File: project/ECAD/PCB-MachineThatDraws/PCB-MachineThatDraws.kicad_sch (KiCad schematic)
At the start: 29 parts, among them J1 SD_Card_Device, J10 Conn_02x03_Odd_Even, J11 Conn_02x03_Odd_Even, J2 SDA/SCL/VCC/GND, J3 Switch, J4 Limit_Switch_X, J5 Moteur, J6 Moteur, J7 Barrel_Jack_Switch, J8 Screw_Terminal_01x02, J9 Servo, U1 ESP32-S3-UNO, U2 R-78E5.0-1.0

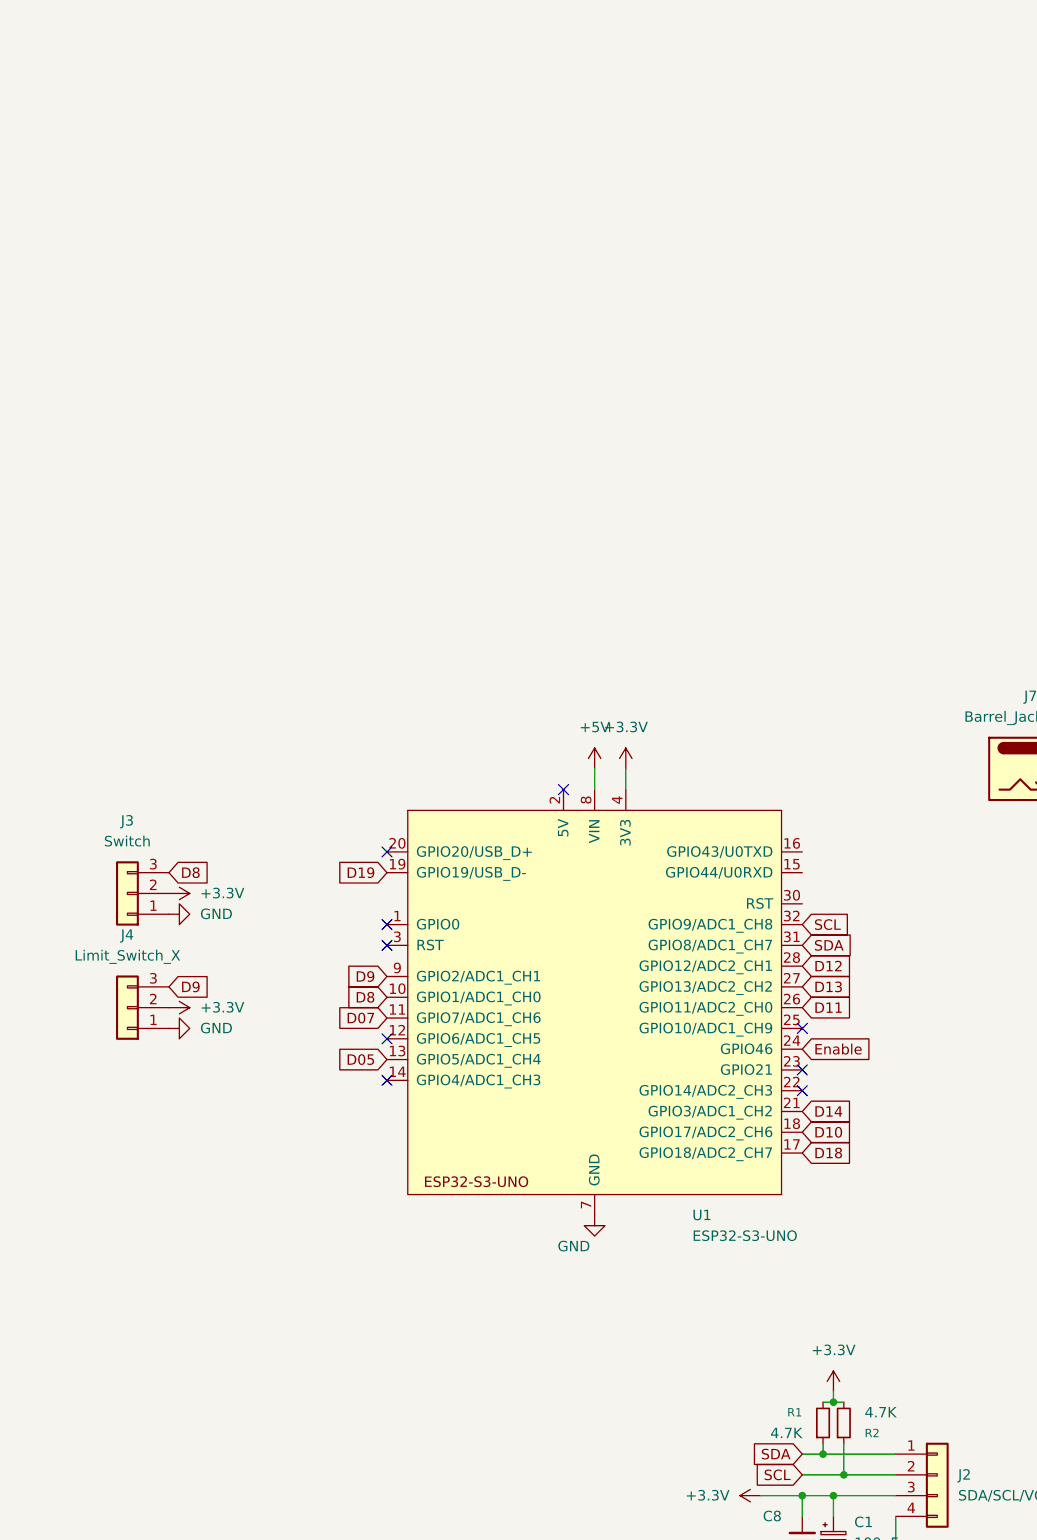
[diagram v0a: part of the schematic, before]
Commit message: new
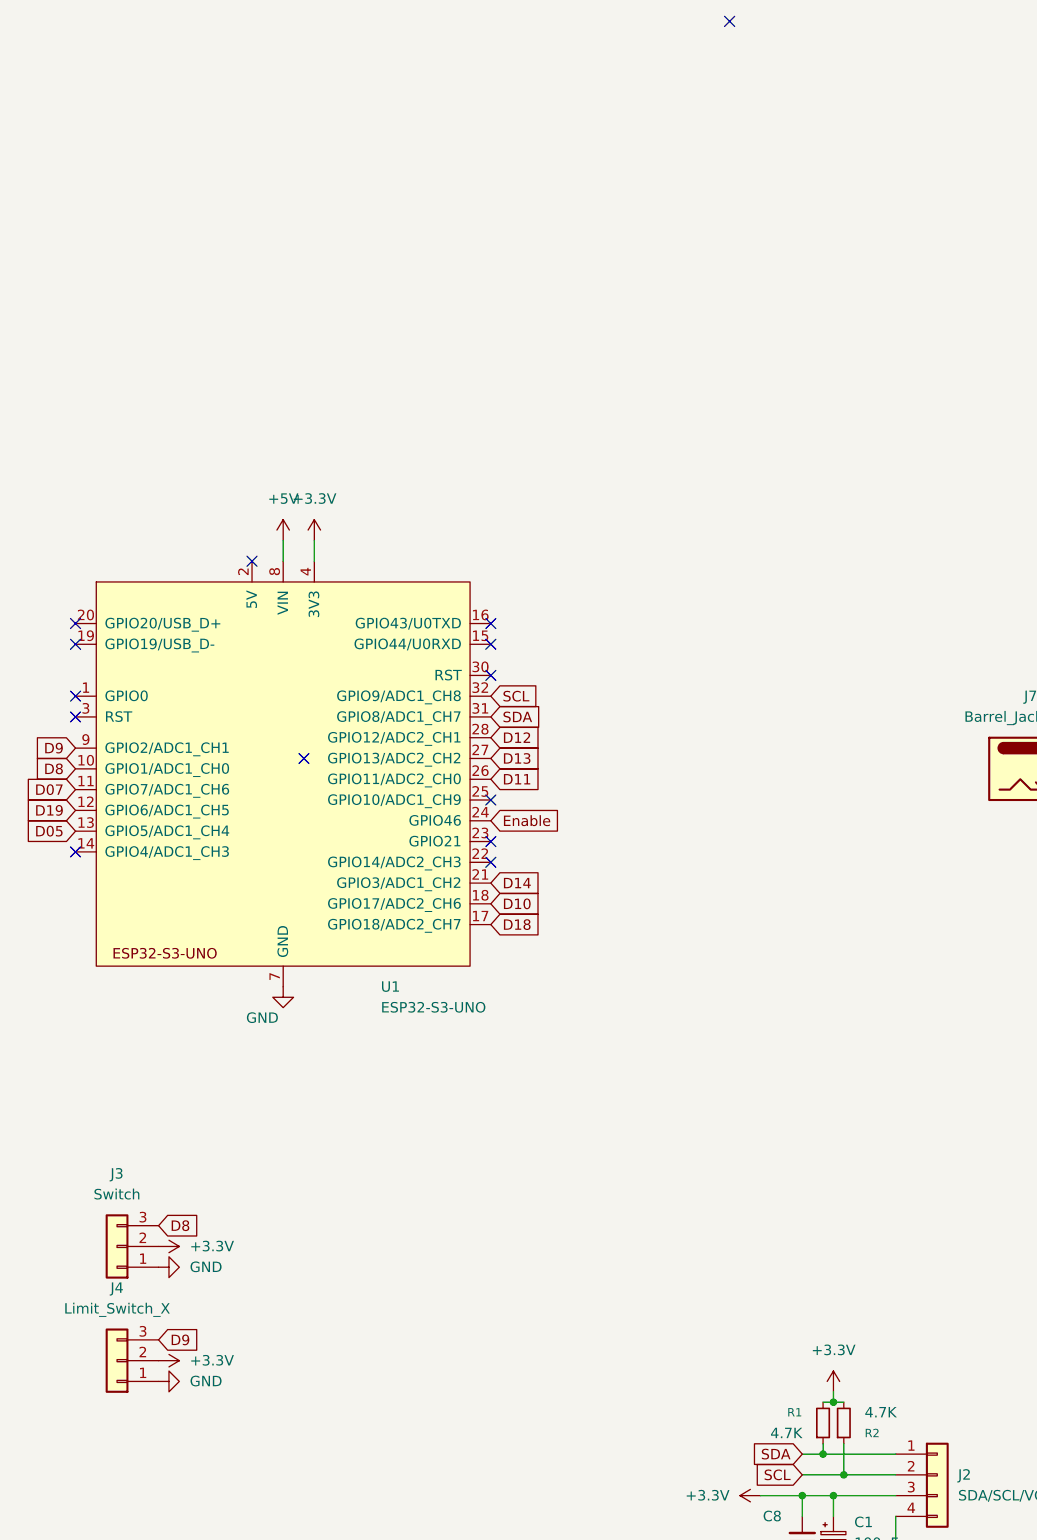
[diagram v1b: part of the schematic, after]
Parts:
- J2, J5, J6: footprint Connector_JST:JST_PH_B3B-PH-K_1x04_P2.00mm_Vertical -> Connector:NS-Tech_Grove_1x04_P2mm_Vertical
- U1: footprint PCM_Espressif:ESP32-S3-DevKitC -> makerspace-unilasalle:ESP_S3_UNO
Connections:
- net D19: now also U1.12 (GPIO6/ADC1_CH5); no longer U1.19 (GPIO19/USB_D-)
- no-connect marks 11 -> 16
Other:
- moved on the sheet: J3, J4, U1
